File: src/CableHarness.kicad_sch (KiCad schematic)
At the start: 11 parts

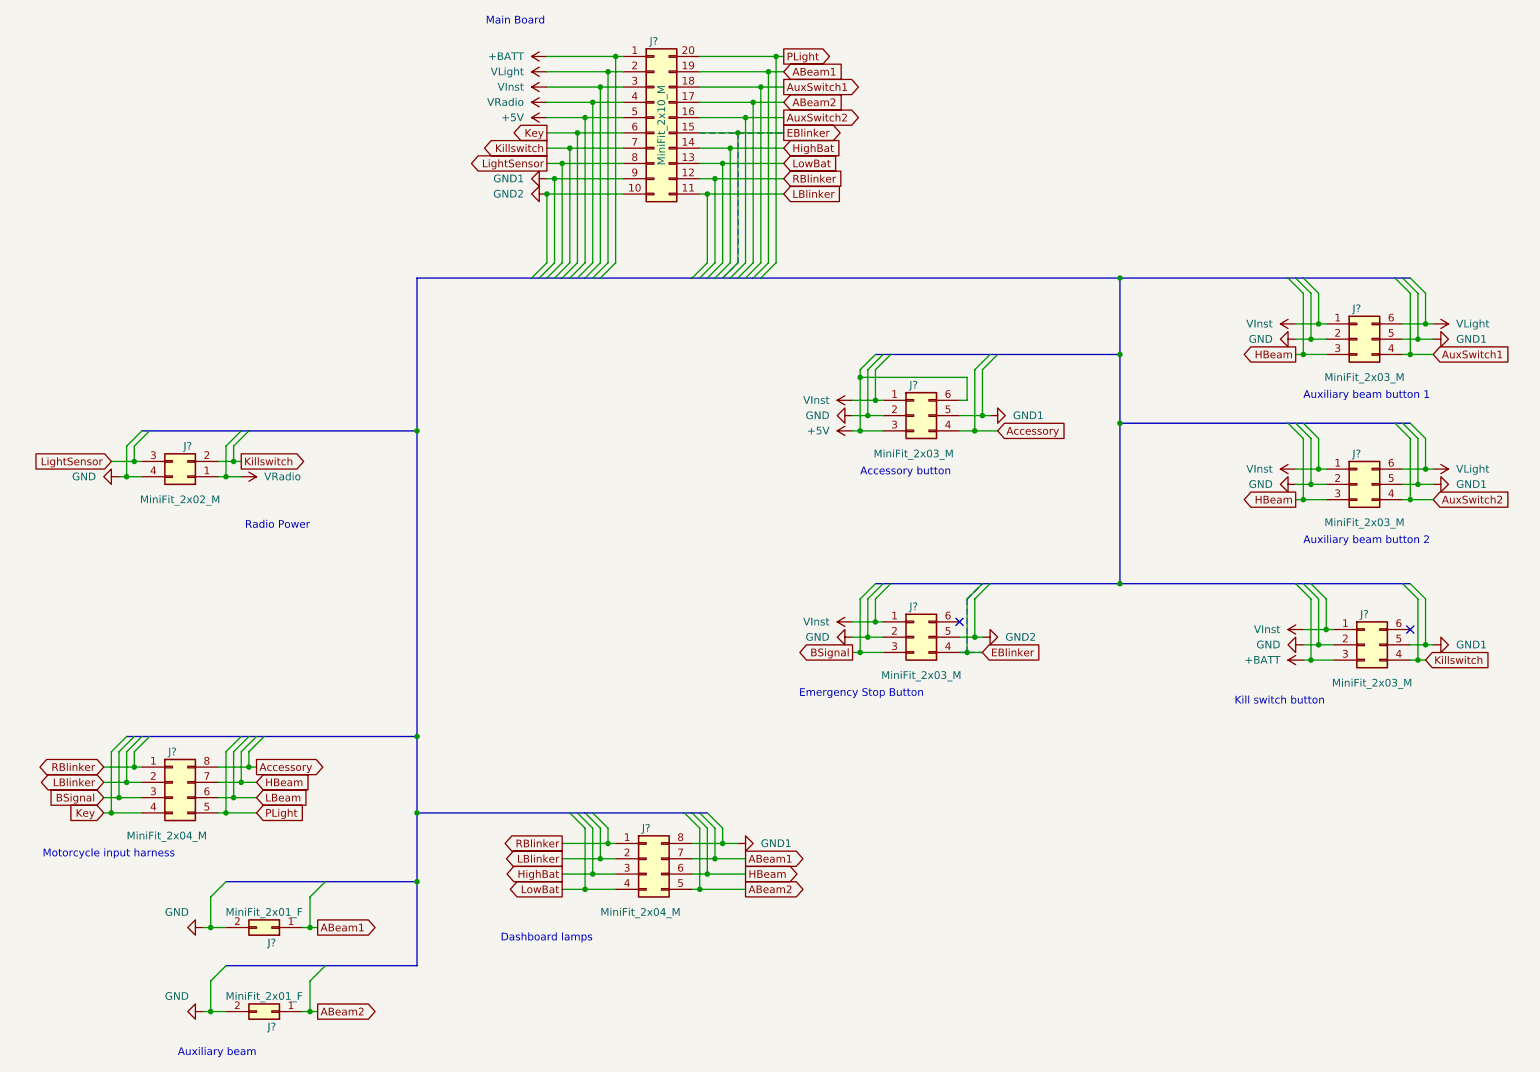
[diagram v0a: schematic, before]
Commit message: Update Schematics design
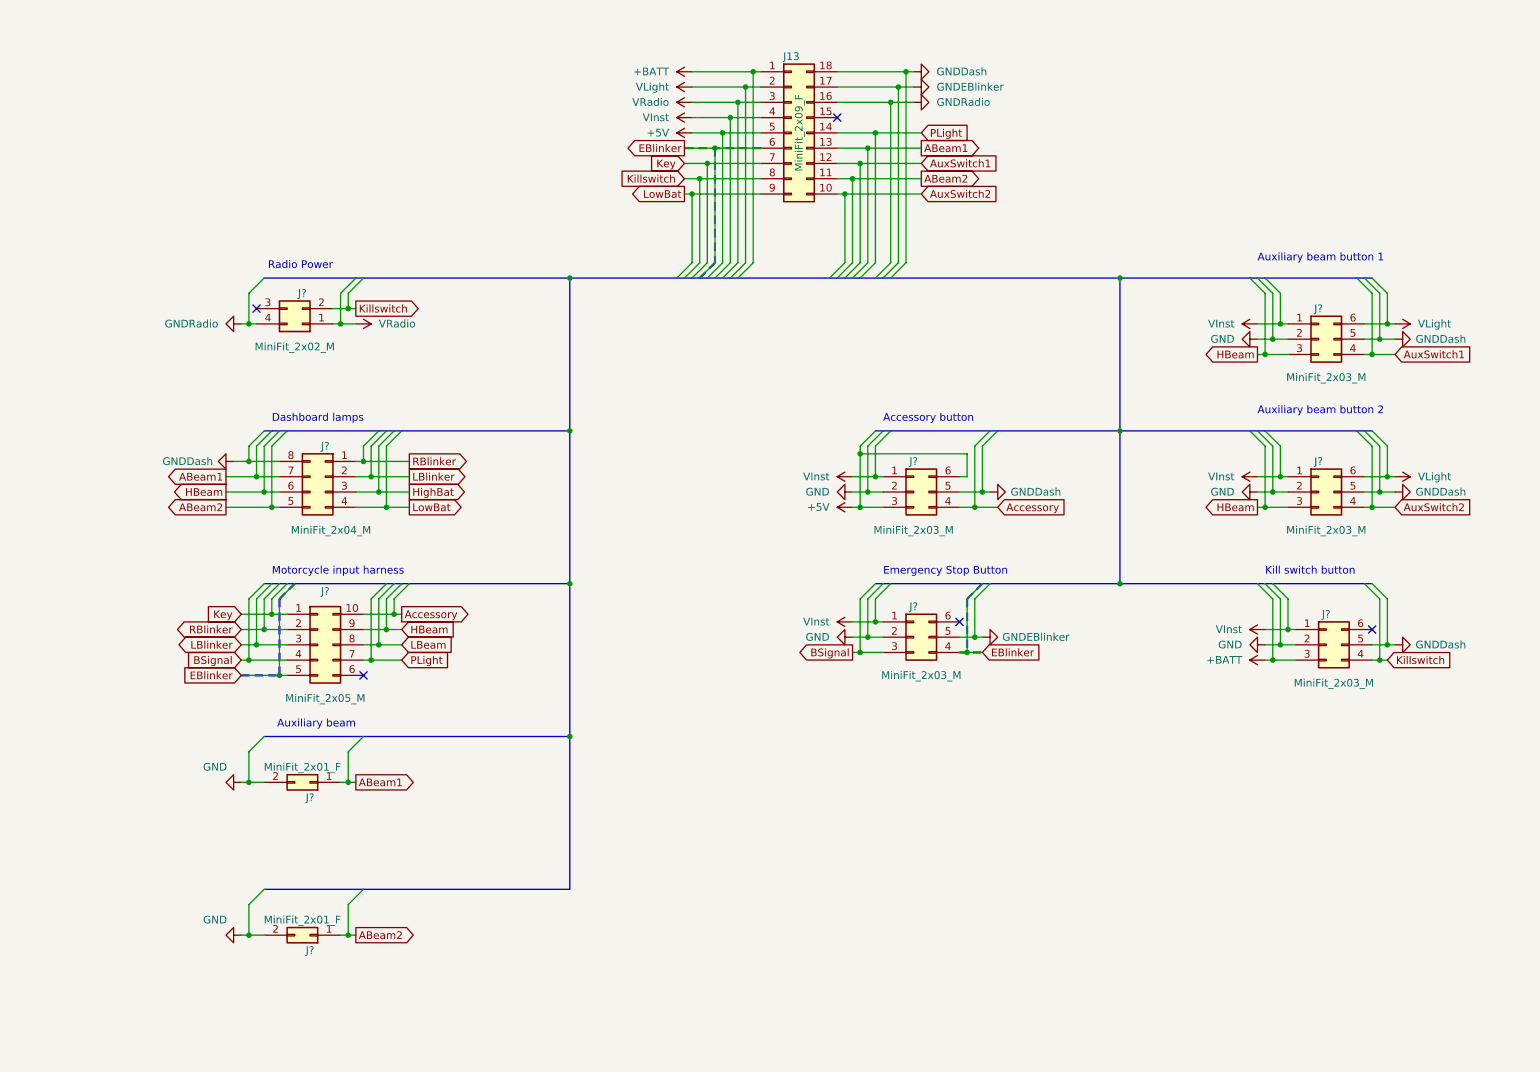
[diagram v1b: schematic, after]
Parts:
- removed J?: MiniFit_2x10_M, Connector_Molex:Molex_Mini-Fit_Jr_5566-20A_2x10_P4.20mm_Vertical, symbol Connector_Generic:Conn_02x10_Counter_Clockwise
- removed J?: MiniFit_2x04_M, Connector_Molex:Molex_Mini-Fit_Jr_5566-08A_2x04_P4.20mm_Vertical, symbol Connector_Generic:Conn_02x04_Counter_Clockwise
- added J13: MiniFit_2x09_F, Connector_Molex:Molex_Mini-Fit_Jr_5566-18A_2x09_P4.20mm_Vertical, symbol Connector_Generic:Conn_02x09_Counter_Clockwise
- added J?: MiniFit_2x05_M, Connector_Molex:Molex_Mini-Fit_Jr_5566-10A_2x05_P4.20mm_Vertical, symbol Connector_Generic:Conn_02x05_Counter_Clockwise
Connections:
- net +5V: now also J13.5 (Pin_5)
- net +BATT: now also J13.1 (Pin_1)
- net ABeam1: now also J13.13 (Pin_13)
- net ABeam2: now also J13.11 (Pin_11)
- net Accessory: now also J?.10 (Pin_10)
- net AuxSwitch1: now also J13.12 (Pin_12)
- net AuxSwitch2: now also J13.10 (Pin_10)
- net BSignal: now also J?.4 (Pin_4)
- net EBlinker: now also J13.6 (Pin_6), J?.5 (Pin_5)
- net GND: no longer J?.4 (Pin_4)
- net HBeam: now also J?.9 (Pin_9)
- net Key: now also J13.7 (Pin_7), J?.1 (Pin_1)
- net Killswitch: now also J13.8 (Pin_8)
- net LBeam: now also J?.8 (Pin_8)
- net LBlinker: now also J?.3 (Pin_3)
- net LowBat: now also J13.9 (Pin_9)
- net PLight: now also J13.14 (Pin_14), J?.7 (Pin_7)
- net RBlinker: now also J?.2 (Pin_2)
- net VInst: now also J13.4 (Pin_4)
- net VLight: now also J13.2 (Pin_2)
- net VRadio: now also J13.3 (Pin_3)
- net GND1 renamed GNDDash
- net GNDDash: now also J13.18 (Pin_18)
- net GND2 renamed GNDEBlinker
- net GNDEBlinker: now also J13.17 (Pin_17)
- net LightSensor: no longer names the net of J?.3 (Pin_3)
- new net GNDRadio: J13.16 (Pin_16), J?.4 (Pin_4)
- no-connect marks 2 -> 5
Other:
- note removed: "Main Board"
- moved on the sheet: J?
